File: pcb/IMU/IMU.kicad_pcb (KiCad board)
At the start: 2 copper layers, 30 x 40 mm, 18 parts, among them J1 Pin Bus, U1 ICM-20948, U3 MIC5365-1.8YC5

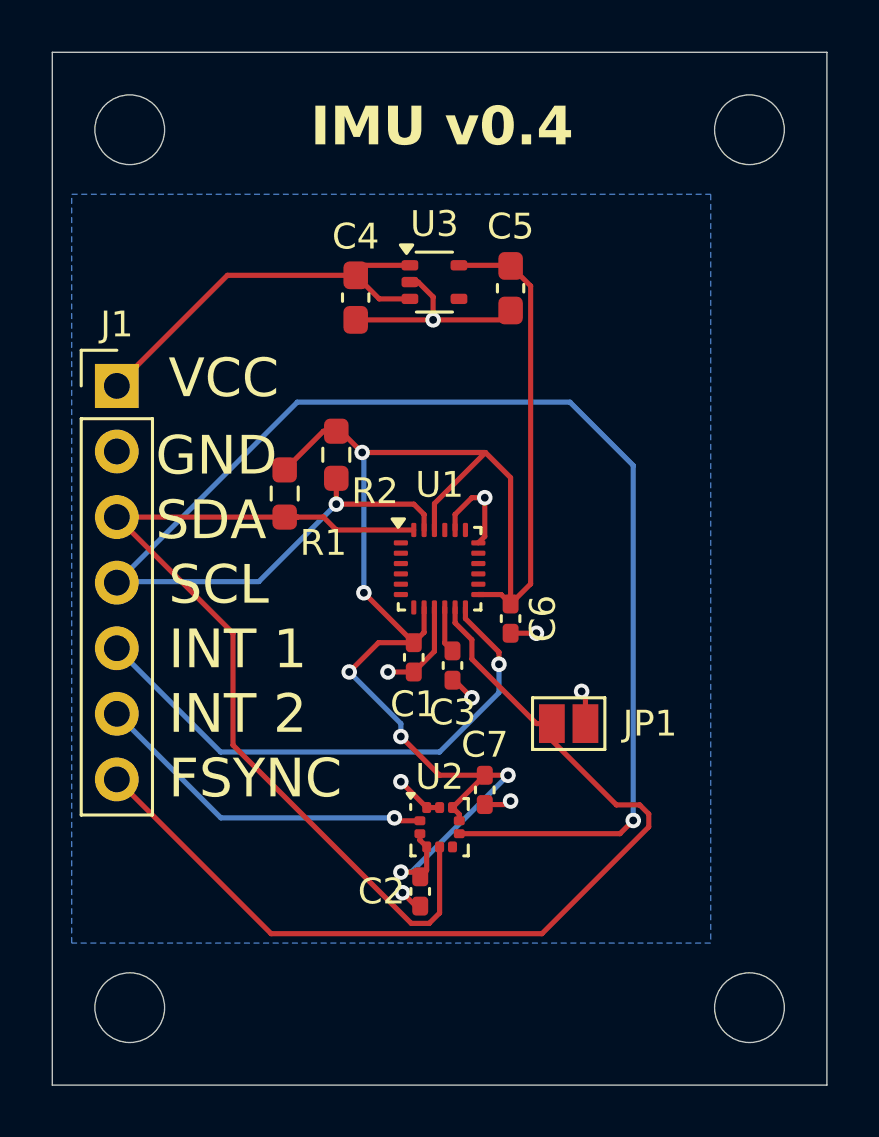
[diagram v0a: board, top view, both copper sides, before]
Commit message: IMU v0.5
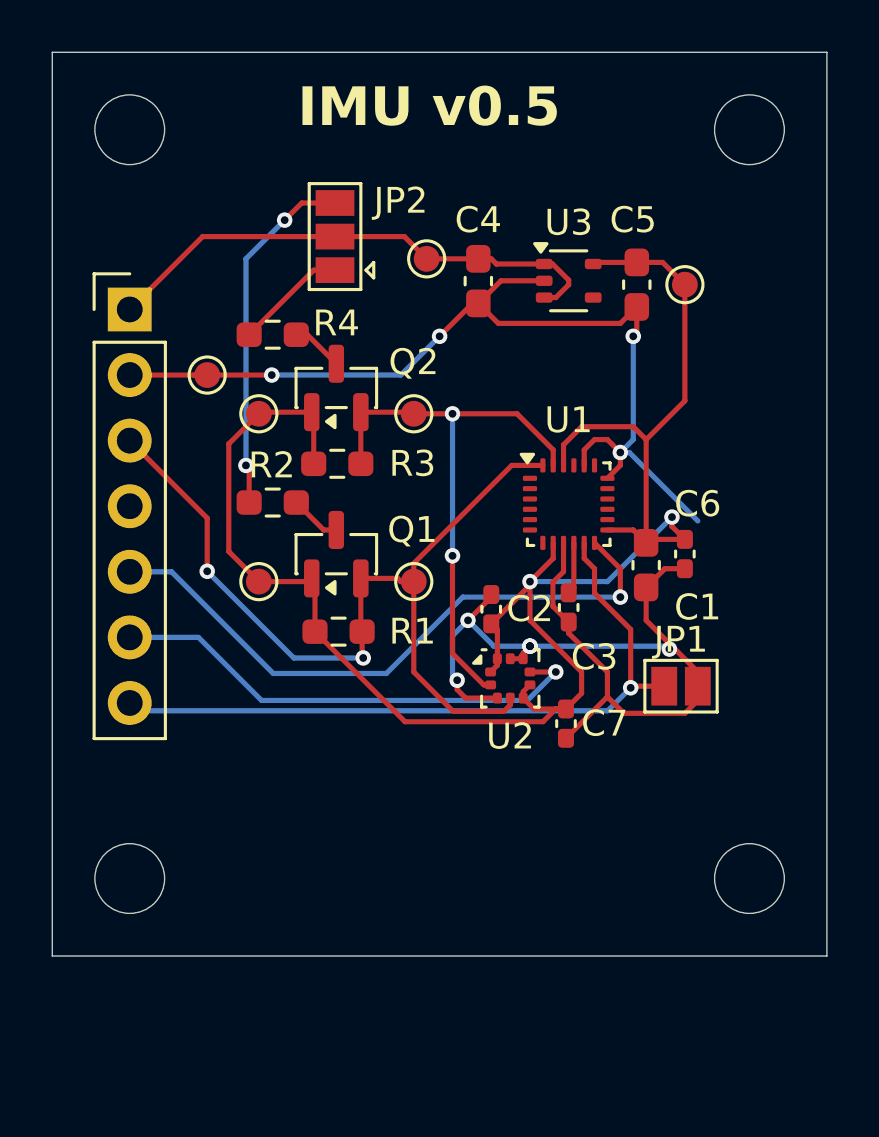
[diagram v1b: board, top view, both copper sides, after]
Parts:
- added JP2: SolderJumper_3_Open, Jumper:SolderJumper-3_P1.3mm_Open_Pad1.0x1.5mm, F.Cu at (145.9, 87.1)
- added Q1: BSS84, Package_TO_SOT_SMD:SOT-23, F.Cu at (146.0, 99.4)
- added Q2: BSS84, Package_TO_SOT_SMD:SOT-23, F.Cu at (146.0, 93.0)
- added R3: 2.2k, Resistor_SMD:R_0603_1608Metric_Pad0.98x0.95mm_HandSolder, F.Cu at (146.0, 95.9)
- added R4: 2.2k, Resistor_SMD:R_0603_1608Metric_Pad0.98x0.95mm_HandSolder, F.Cu at (143.5, 90.9)
- added TP1: TestPoint, TestPoint:TestPoint_Pad_D1.0mm, F.Cu at (143.0, 100.5)
- added TP2: TestPoint, TestPoint:TestPoint_Pad_D1.0mm, F.Cu at (149.0, 100.5)
- added TP3: TestPoint, TestPoint:TestPoint_Pad_D1.0mm, F.Cu at (149.5, 88.0)
- added TP4: TestPoint, TestPoint:TestPoint_Pad_D1.0mm, F.Cu at (159.5, 89.0)
- added TP5: TestPoint, TestPoint:TestPoint_Pad_D1.0mm, F.Cu at (141.0, 92.5)
- added TP6: TestPoint, TestPoint:TestPoint_Pad_D1.0mm, F.Cu at (149.0, 94.0)
- added TP7: TestPoint, TestPoint:TestPoint_Pad_D1.0mm, F.Cu at (143.0, 94.0)
- C1: value 0.1uf -> 1uf; footprint Capacitor_SMD:C_0402_1005Metric_Pad0.74x0.62mm_HandSolder -> Capacitor_SMD:C_0603_1608Metric_Pad1.08x0.95mm_HandSolder
- moved C2 11.3 mm to (152.0, 101.6), turned to 90 degrees
- moved C1 9.68 mm to (158.0, 99.9)
- moved C6 7.20 mm to (159.5, 99.4)
- moved U2 6.38 mm to (152.7, 104.2)
- moved R1 5.74 mm to (146.1, 102.4), turned to 0 degrees
- moved U1 5.59 mm to (155.0, 97.5)
- moved U3 5.20 mm to (155.0, 88.8)
- moved C3 5.03 mm to (155.0, 101.5)
- moved REF** 5.00 mm to (138.0, 112.0)
- moved REF** 5.00 mm to (162.0, 112.0)
- moved C5 4.89 mm to (157.6, 89.0)
- moved C4 4.79 mm to (151.5, 88.9)
- moved JP1 4.59 mm to (159.3, 104.5)
- moved C7 4.06 mm to (154.9, 106.0)
- moved R2 3.08 mm to (143.5, 97.4), turned to 0 degrees
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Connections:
- net Net-(J1-Pin_1) renamed /VIN
- R2 pad 1: /1.8v -> Net-(JP2-B)
- R2 pad 2: /SCL -> Net-(Q1-D)
- U1 pad 7: unconnected-(U1-AUX_CL-Pad7) -> (no net)
- U2 pad 3: (no net) -> GND
- U2 pad 8: (no net) -> GND
- U2 pad 9: (no net) -> GND
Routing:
- net GND: track 23.2 -> 74.3 mm
- net /SCL: track 59.5 -> 21.9 mm
- net Net-(JP2-B): track 0.00 -> 13.8 mm, vias 0 -> 2
- net /FSYNC: track 37.3 -> 27.7 mm, vias 0 -> 1
- net /INT2: track 13.5 -> 19.0 mm
- net Net-(JP2-A): track 0.00 -> 4.36 mm
- net /VIN: track 16.0 -> 20.2 mm
- net /1.8v: track 67.8 -> 71.9 mm, vias 6 -> 2
- net /INT1: track 21.3 -> 24.4 mm
- net Net-(Q2-D): track 0.00 -> 2.02 mm
- net Net-(Q1-D): track 0.00 -> 1.99 mm
- net /SDA: track 36.0 -> 34.5 mm, vias 0 -> 2
- removed copper zone on B.Cu, net GND
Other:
- board size 30 x 40 mm -> 30 x 35 mm
- board text added: "IMU v0.5"
- board text removed: "FSYNC"
- board text removed: "GND"
- board text removed: "IMU v0.4"
- board text removed: "INT 1"
- board text removed: "INT 2"
- board text removed: "SCL"
- board text removed: "SDA"
- board text removed: "VCC"
